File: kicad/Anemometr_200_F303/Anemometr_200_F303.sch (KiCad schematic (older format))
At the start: 44 parts, among them J1 Conn_01x01_Female, J10 USB_B_Micro, J11 Conn_01x01_Female, J12 Conn_01x01_Female, J13 Conn_01x01_Female, J14 Conn_01x01_Female, J15 Conn_01x01_Female, J16 Conn_01x01_Female, J17 Conn_01x01_Female, J18 Conn_01x01_Female, J19 Conn_01x01_Female, J2 Conn_01x01_Female, J20 Conn_01x01_Female, J21 Conn_01x01_Female, J22 Conn_01x01_Female, J23 Conn_01x01_Female, J24 Conn_01x01_Female, J25 Conn_01x01_Female, J26 Conn_01x01_Female, J27 Conn_01x01_Female, J3 Conn_01x01_Female, J4 Conn_01x01_Female, J5 Conn_01x01_Female, J6 Conn_01x01_Female, U1 AP1117-33, U2 STM32F303CCTx, U3 CH340C, Y1 16MHz

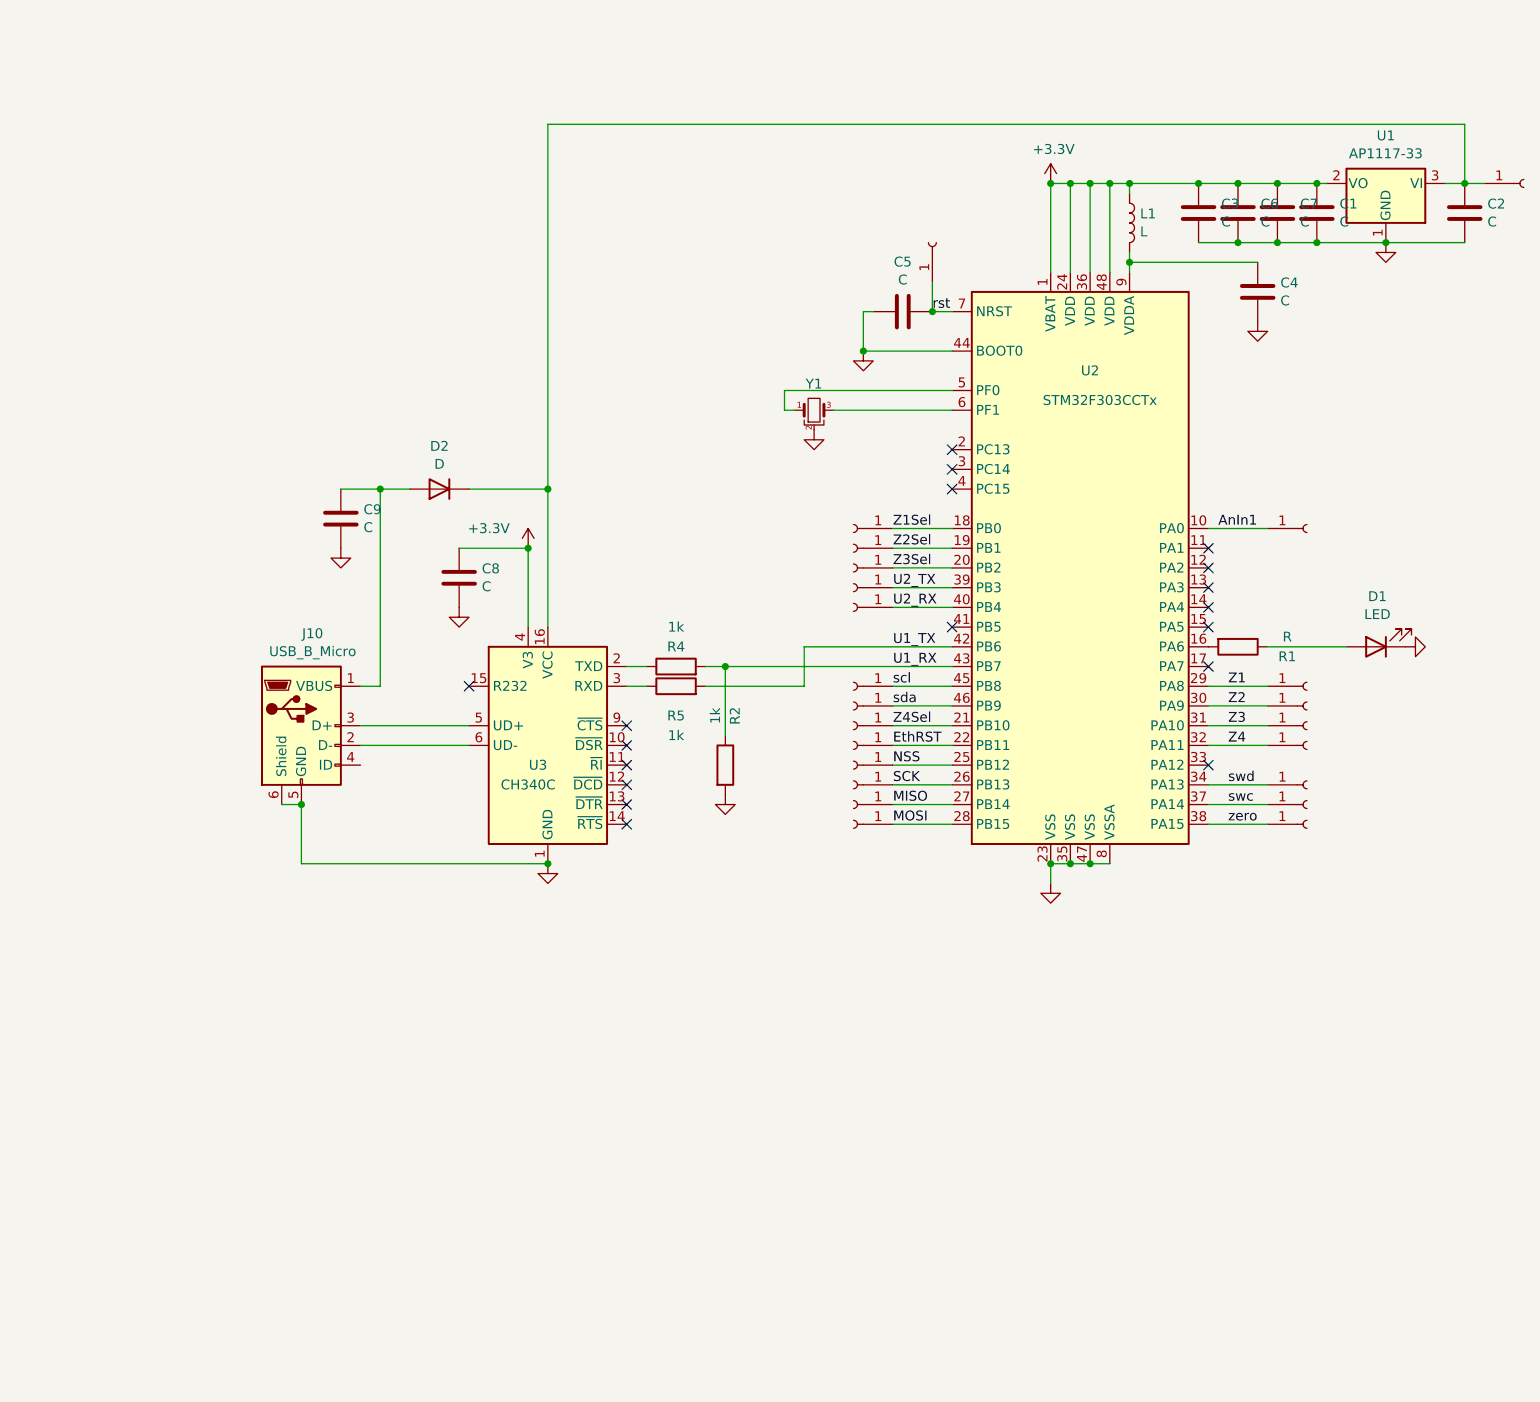
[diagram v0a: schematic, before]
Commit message: изменено:      Documents/matLab/convData.m 	изменено:      kicad/Anemometr_200_F303/Anemometr_200_F303-cache.lib 	изменено:      kicad/Anemometr_200_F303/Anemometr_200_F303.kicad_pcb 	изменено:      kicad/Anemometr_200_F303/Anemometr_200_F303.kicad_pcb-bak 	изменено:      kicad/Anemometr_200_F303/Anemometr_200_F303.sch 	изменено:      kicad/Anemometr_200_F303/Anemometr_200_F303.sch-bak 	изменено:      kicad/Anemometr_200_F303/fp-info-cache 	изменено:      stm32cubeide/Anemometer_200_F303/Anemometer_200_F303.ioc 	новый файл:    stm32cubeide/Anemometer_200_F303/Core/Inc/FFTImplementationCallback.h 	изменено:      stm32cubeide/Anemometer_200_F303/Core/Inc/main.h 	новый файл:    stm32cubeide/Anemometer_200_F303/Core/Inc/maxEnvHilbert.h 	новый файл:    stm32cubeide/Anemometer_200_F303/Core/Inc/maxEnvHilbert_data.h 	новый файл:    stm32cubeide/Anemometer_200_F303/Core/Inc/maxEnvHilbert_terminate.h 	новый файл:    stm32cubeide/Anemometer_200_F303/Core/Inc/rt_nonfinite.h 	новый файл:    stm32cubeide/Anemometer_200_F303/Core/Inc/rtwtypes.h 	новый файл:    stm32cubeide/Anemometer_200_F303/Core/Inc/tmwtypes.h 	новый файл:    stm32cubeide/Anemometer_200_F303/Core/Src/FFTImplementationCallback.c 	изменено:      stm32cubeide/Anemometer_200_F303/Core/Src/main.c 	новый файл:    stm32cubeide/Anemometer_200_F303/Core/Src/maxEnvHilbert.c 	новый файл:    stm32cubeide/Anemometer_200_F303/Core/Src/maxEnvHilbert_data.c 	новый файл:    stm32cubeide/Anemometer_200_F303/Core/Src/maxEnvHilbert_terminate.c 	новый файл:    stm32cubeide/Anemometer_200_F303/Core/Src/rt_nonfinite.c 	изменено:      stm32cubeide/Anemometer_200_F303/Core/Src/stm32f3xx_hal_msp.c 	изменено:      stm32cubeide/Anemometer_200_F303/Core/Src/stm32f3xx_it.c 	изменено:      stm32cubeide/Anemometer_200_F303/Debug/Anemometer_200_F303.elf 	изменено:      stm32cubeide/Anemometer_200_F303/Debug/Anemometer_200_F303.list 	изменено:      stm32cubeide/Anemometer_200_F303/Debug/Anemometer_200_F303.map 	изменено:      stm32cubeide/Anemo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
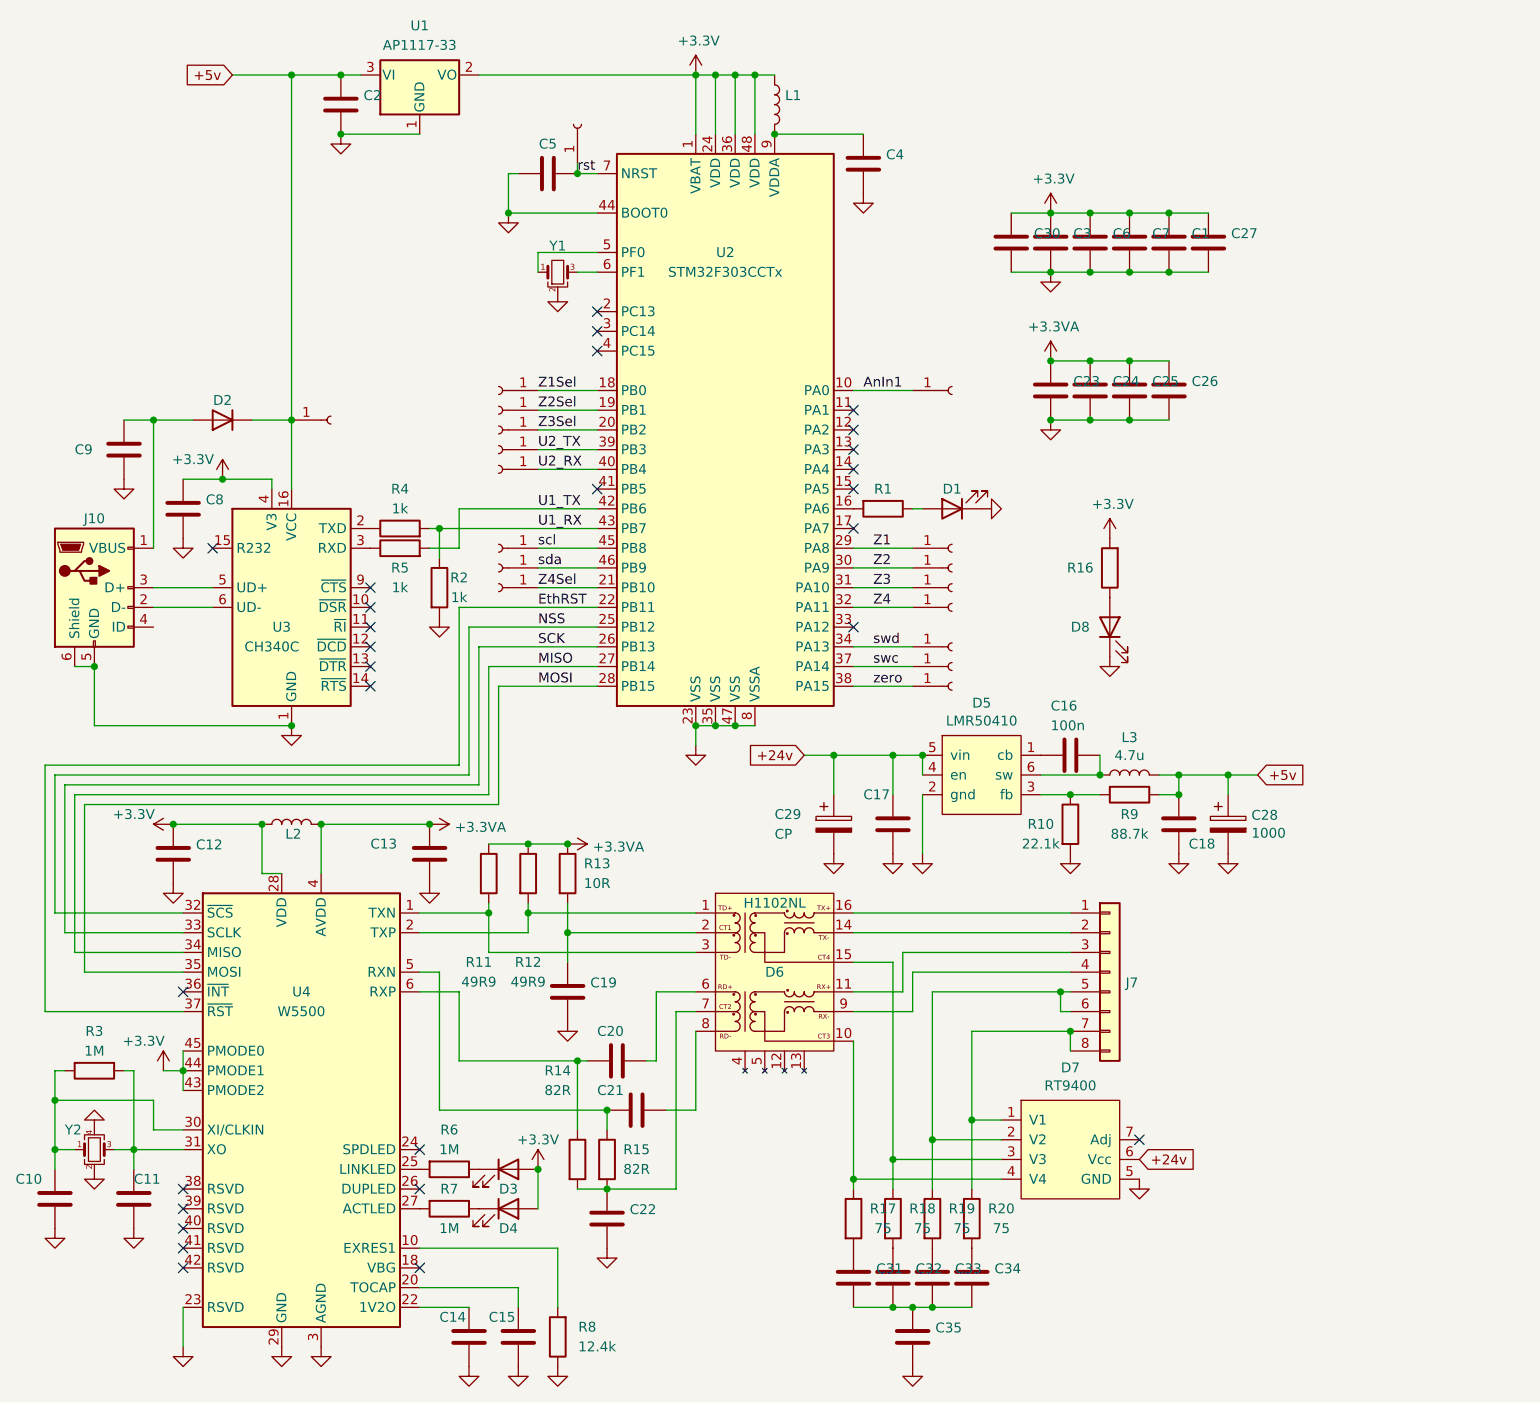
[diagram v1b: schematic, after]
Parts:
- removed J18, J20, J21, J22, J24: Conn_01x01_Female, My-library:mini_conn, symbol Connector:Conn_01x01_Female
- added C10, C11, C13, C23, C24, C25, C26, C27: C, Capacitor_SMD:C_0402_1005Metric, symbol Device:C
- added C12: C, Capacitor_SMD:C_0603_1608Metric, symbol Device:C
- added C14, C22: 10n, Capacitor_SMD:C_0402_1005Metric, symbol Device:C
- added C15: 4.7u, Capacitor_SMD:C_0402_1005Metric, symbol Device:C
- added C16: 100n, Capacitor_SMD:C_0805_2012Metric, symbol Device:C
- added C17, C18, C30: C, Capacitor_SMD:C_0805_2012Metric, symbol Device:C
- added C19: 22n, Capacitor_SMD:C_0402_1005Metric, symbol Device:C
- added C20, C21, C31, C32, C33, C34: 6.8n, Capacitor_SMD:C_0402_1005Metric, symbol Device:C
- added C28: 1000, Capacitor_Tantalum_SMD:CP_EIA-7343-15_Kemet-W, symbol Device:CP
- added C29: CP, Capacitor_Tantalum_SMD:CP_EIA-7343-15_Kemet-W, symbol Device:CP
- added C35: 6.8n, Capacitor_SMD:C_1206_3216Metric, symbol Device:C
- added D3, D4, D8: LED, LED_SMD:LED_0603_1608Metric, symbol Device:LED
- added D5: LMR50410, Package_TO_SOT_SMD:SOT-23-6, symbol My_Library:LMR50410
- added D6: H1102NL, My-library:H1102N, symbol My_Library:H1102NL
- added D7: RT9400, My-library:TR9400, symbol My_Library:RT9400
- added J7: Conn_01x08, Connector_JST:JST_SH_BM08B-SRSS-TB_1x08-1MP_P1.00mm_Vertical, symbol Connector_Generic:Conn_01x08
- added L2: L, Inductor_SMD:L_0805_2012Metric, symbol Device:L
- added L3: 4.7u, Inductor_SMD:L_Abracon_ASPI-0630LR, symbol Device:L
- added R10: 22.1k, Resistor_SMD:R_0603_1608Metric, symbol Device:R
- added R11, R12: 49R9, Resistor_SMD:R_0402_1005Metric, symbol Device:R
- added R13: 10R, Resistor_SMD:R_0402_1005Metric, symbol Device:R
- added R14, R15: 82R, Resistor_SMD:R_0402_1005Metric, symbol Device:R
- added R16: 1k, Resistor_SMD:R_0603_1608Metric, symbol Device:R
- added R17, R18, R19, R20: 75, Resistor_SMD:R_0402_1005Metric, symbol Device:R
- added R3, R6, R7: 1M, Resistor_SMD:R_0402_1005Metric, symbol Device:R
- added R8: 12.4k, Resistor_SMD:R_0402_1005Metric, symbol Device:R
- added R9: 88.7k, Resistor_SMD:R_0603_1608Metric, symbol Device:R
- added U4: W5500, Package_QFP:LQFP-48_7x7mm_P0.5mm, symbol Interface_Ethernet:W5500
- added Y2: Crystal_GND24_Small, Crystal:Crystal_SMD_SeikoEpson_FA238-4Pin_3.2x2.5mm, symbol Device:Crystal_GND24_Small
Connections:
- net +3V3: now also C12.1, C27.1, C30.1, D3.2 (A), D4.2 (A), L2.1, R16.2, U4.28 (VDD), U4.43 (PMODE2), U4.44 (PMODE1), U4.45 (PMODE0)
- net EthRST: now also U4.37 (~RST)
- net GND: now also C10.2, C11.2, C12.2, C13.2, C14.2, C15.2, C17.2, C18.2, C19.2, C22.2, C23.2, C24.2, C25.2, C26.2, C27.2, C28.2, C29.2, C30.2, C35.2, D5.2 (gnd), D7.5 (GND), D8.1 (K), R10.2, R8.1, U4.14 (AGND), U4.16 (AGND), U4.19 (AGND), U4.23 (RSVD), U4.29 (GND), U4.3 (AGND), U4.48 (AGND), U4.9 (AGND), Y2.2, Y2.4
- net MISO: now also U4.34 (MISO)
- net MOSI: now also U4.35 (MOSI)
- net NSS: now also U4.32 (~SCS)
- net SCK: now also U4.33 (SCLK)
- net +5v: now reaches C2.1, D2.1 (K), J1.1 (Pin_1), U1.3 (VI), U3.16 (VCC)
- net +5v: now also C18.1, C28.1, L3.2, R9.1
- new net: D8.2 (A), R16.1
- new net: D6.10, D7.4 (V4), R17.1
- new net: C31.1, R17.2
- new net: D6.15, D7.3 (V3), R18.1
- new net: C32.1, R18.2
- new net: D7.2 (V2), J7.5 (Pin_5), J7.6 (Pin_6), R19.1
- new net: C33.1, R19.2
- new net: D7.1 (V1), J7.7 (Pin_7), J7.8 (Pin_8), R20.1
- new net: C34.1, R20.2
- new net: C31.2, C32.2, C33.2, C34.2, C35.1
- new net: D6.3, R11.2, U4.1 (TXN)
- new net: R8.2, U4.10 (EXRES1)
- new net: D6.1, R12.2, U4.2 (TXP)
- new net: C15.1, U4.20 (TOCAP)
- new net: C14.1, U4.22 (1V2O)
- new net: R6.2, U4.25 (LINKLED)
- new net: R7.2, U4.27 (ACTLED)
- new net: C10.1, R3.2, U4.30 (XI/CLKIN), Y2.1
- new net: C11.1, R3.1, U4.31 (XO), Y2.3
- new net: C21.2, R15.1, U4.5 (RXN)
- new net: C20.2, R14.1, U4.6 (RXP)
- new net: D3.1 (K), R6.1
- new net: D4.1 (K), R7.1
- new net: D6.11, J7.3 (Pin_3)
- new net: D6.14, J7.2 (Pin_2)
- new net: D6.16, J7.1 (Pin_1)
- new net: C19.1, D6.2, R13.2
- new net: C20.1, D6.6
- new net: C22.1, D6.7, R14.2, R15.2
- new net: C21.1, D6.8
- new net: D6.9, J7.4 (Pin_4)
- new net: C16.2, D5.1 (cb)
- new net: D5.3 (fb), R10.1, R9.2
- new net: C16.1, D5.6 (sw), L3.1
- new net +24v: C17.1, C29.1, D5.4 (en), D5.5 (vin), D7.6 (Vcc)
- new net +3.3VA: C13.1, C23.1, C24.1, C25.1, C26.1, L2.2, R11.1, R12.1, R13.1, U4.11 (AVDD), U4.15 (AVDD), U4.17 (AVDD), U4.21 (AVDD), U4.4 (AVDD), U4.8 (AVDD)
- no-connect marks 18 -> 28
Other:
- moved on the sheet: C1, C2, C3, C4, C5, C6, C7, C8, C9, D1, D2, J10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
